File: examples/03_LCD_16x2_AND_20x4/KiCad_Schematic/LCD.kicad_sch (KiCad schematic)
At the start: 13 parts, among them J1 KIT DIY 5~7W QN8066, U1 LCD 16x02 or 20x04, U2 L78L05_SO8

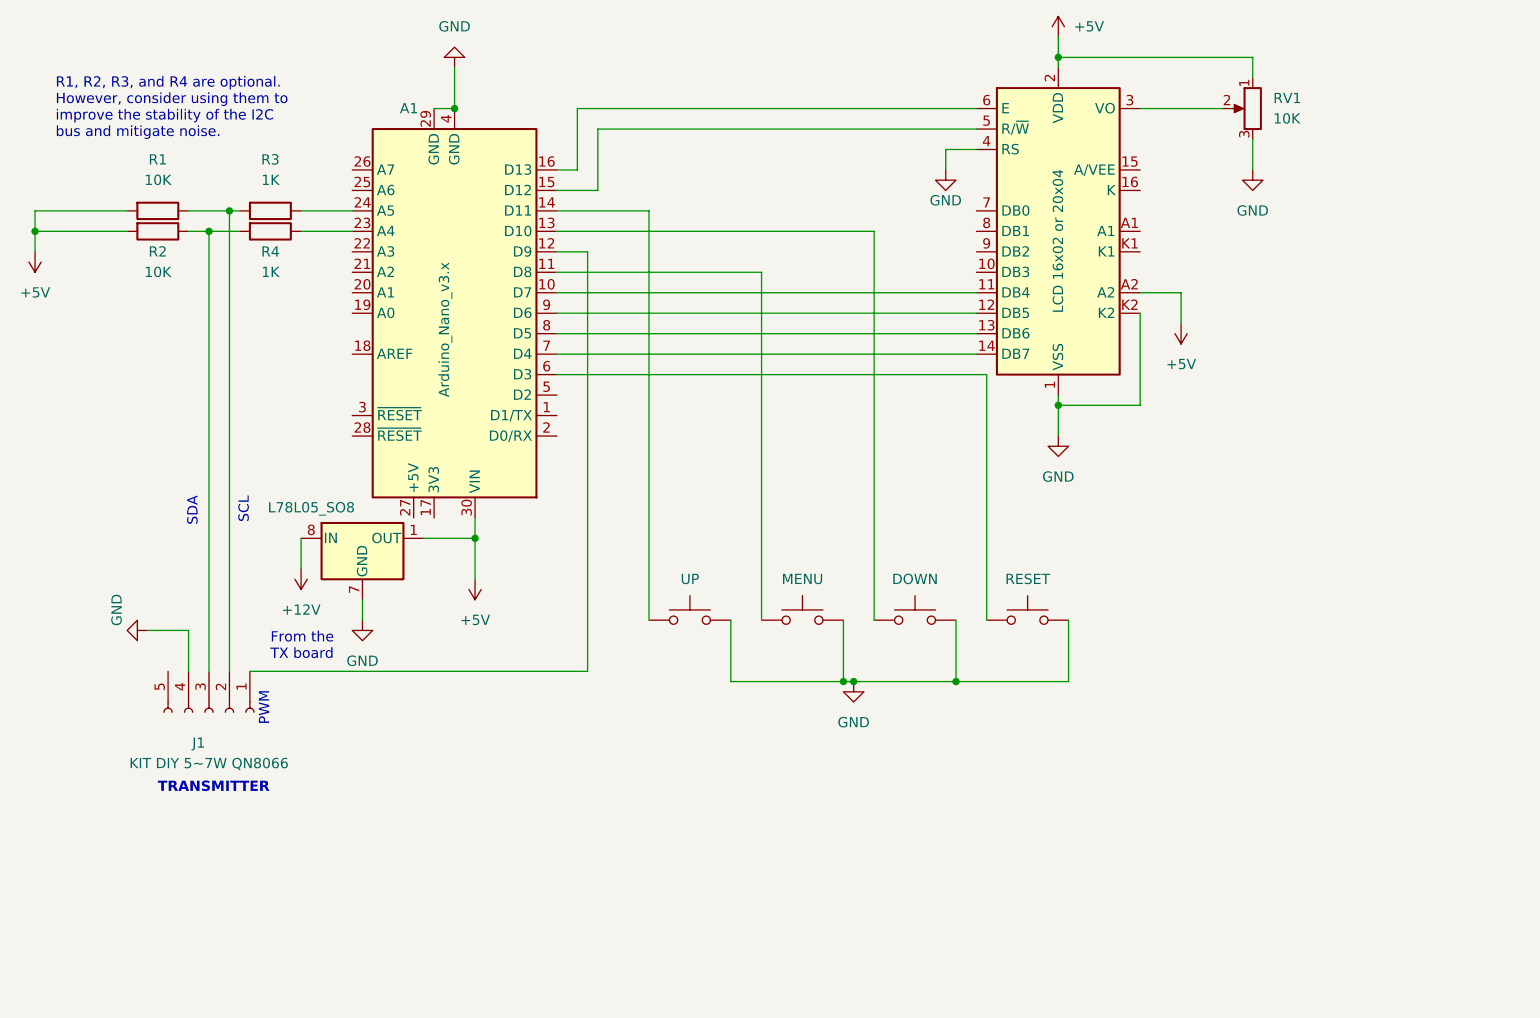
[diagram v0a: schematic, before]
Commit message: Doc
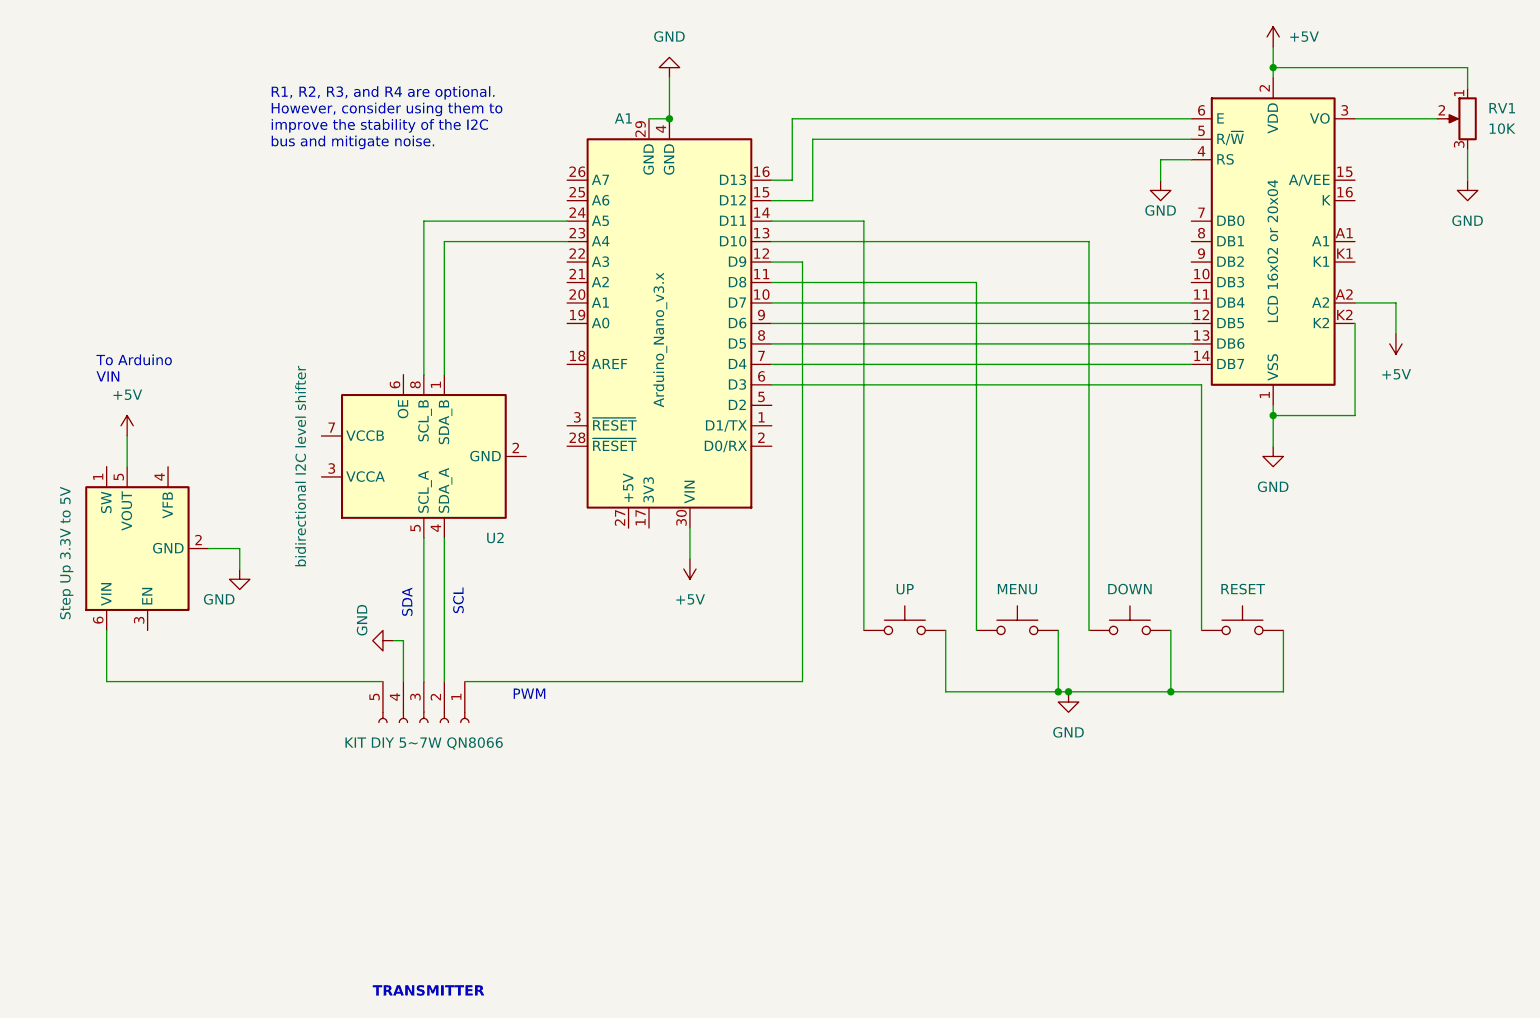
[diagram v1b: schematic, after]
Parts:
- removed R1, R2: 10K, symbol Device:R
- removed R3, R4: 1K, symbol Device:R
- removed U2: L78L05_SO8, Package_SO:SOIC-8_3.9x4.9mm_P1.27mm, symbol Regulator_Linear:L78L05_SO8
- added U2: bidirectional I2C level shifter, symbol Interface:TCA9406DC
- added U3: Step Up 3.3V to 5V, Package_TO_SOT_SMD:SOT-23-6, symbol Regulator_Switching:MCP1640CCH
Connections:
- net +5V: now also U3.5 (VOUT)
- net GND: now also U3.2 (GND)
- net at J1.2 (Pin_2): now also U2.4 (SDA_A)
- net at J1.3 (Pin_3): now also U2.5 (SCL_A)
- net at J1.5 (Pin_5): now also U3.6 (VIN)
- net at A1.24 (A5): now also U2.8 (SCL_B)
- net at A1.23 (A4): now also U2.1 (SDA_B)
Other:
- note added: "To Arduino VIN"
- note removed: "From the TX board"
- moved on the sheet: A1, DOWN, MENU, RESET, RV1, UP
